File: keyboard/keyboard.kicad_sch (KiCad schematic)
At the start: 61 parts, among them J1 Conn_02x12_Odd_Even, SW1 true video, SW10 8, SW11 9, SW12 0, SW13 Break, SW14 delete, SW15 q, SW16 w, SW17 e, SW18 r, SW19 t, SW2 inverted video, SW20 y, SW21 u, SW22 i, SW23 o, SW24 p, SW25 graph, SW26 extended mode, SW27 edit, SW28 a, SW29 s, SW3 1, SW30 d, SW31 f, SW32 g, SW33 h, SW34 j, SW35 k, SW36 l, SW37 enter, SW38 caps shift left, SW39 caps lock, SW4 2, SW40 z, SW41 x, SW42 c, SW43 v, SW44 b, SW45 n, SW46 m, SW47 dot, SW48 caps shift right, SW49 symbol shift left, SW5 3, SW50 semicolon, SW51 quotes, SW52 left, SW53 right, SW54 left space, SW55 right space, SW56 up, SW57 down, SW58 comma, SW59 symbol shift right, SW6 4, SW60 rus-lat, SW7 5, SW8 6, SW9 7

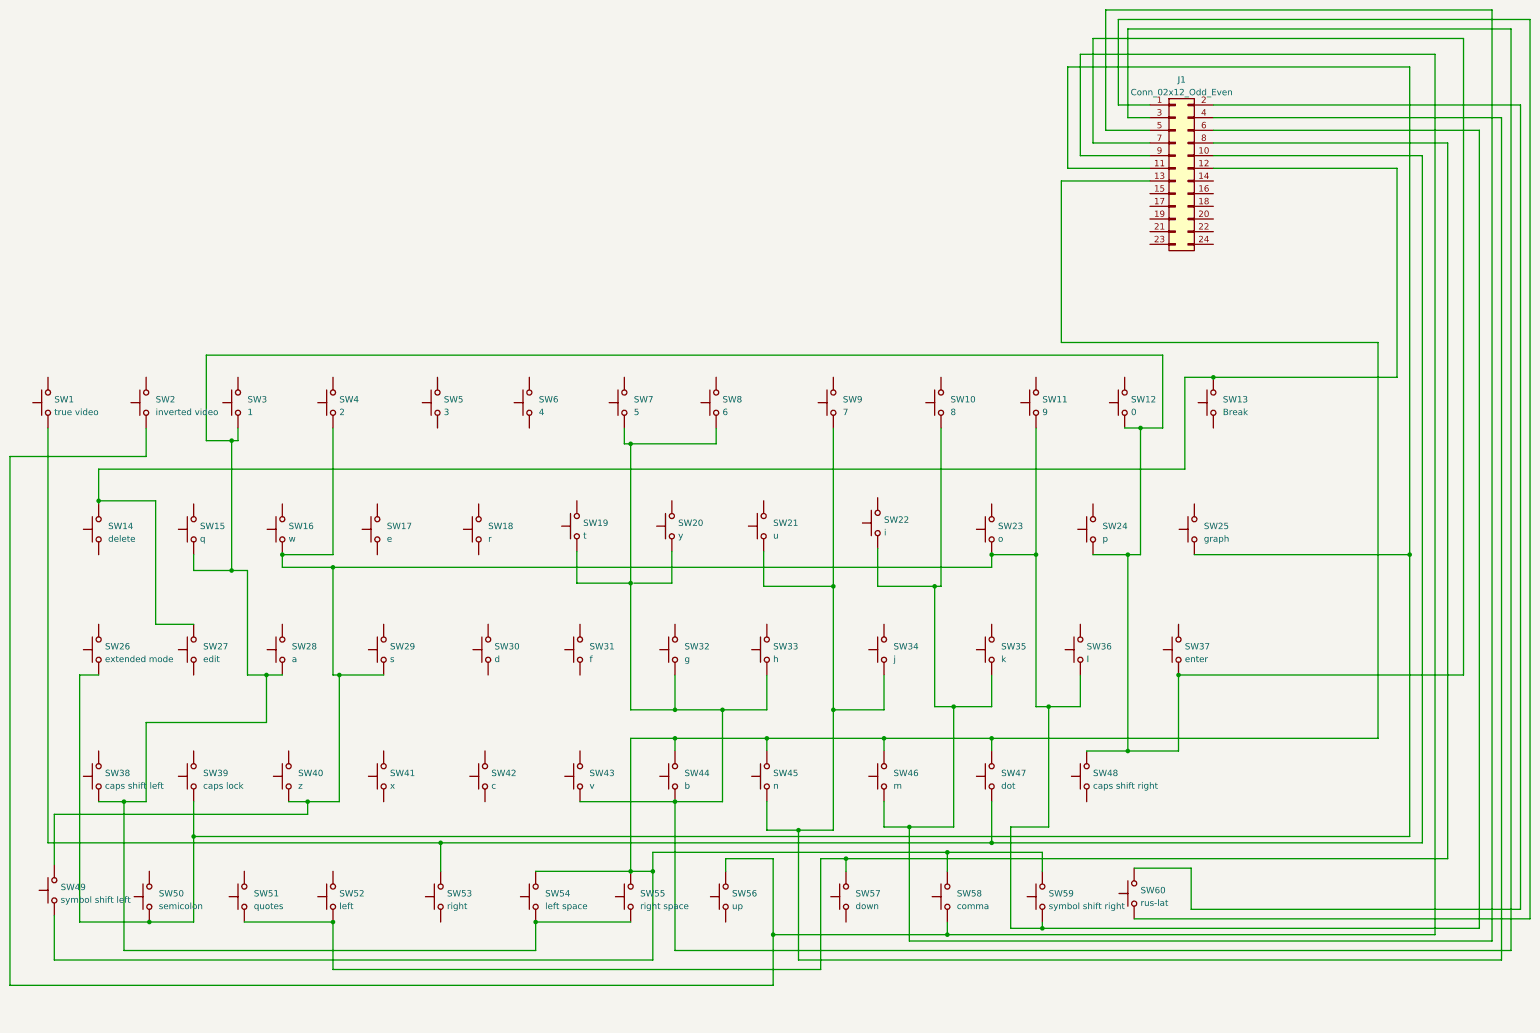
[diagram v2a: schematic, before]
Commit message: Late night update
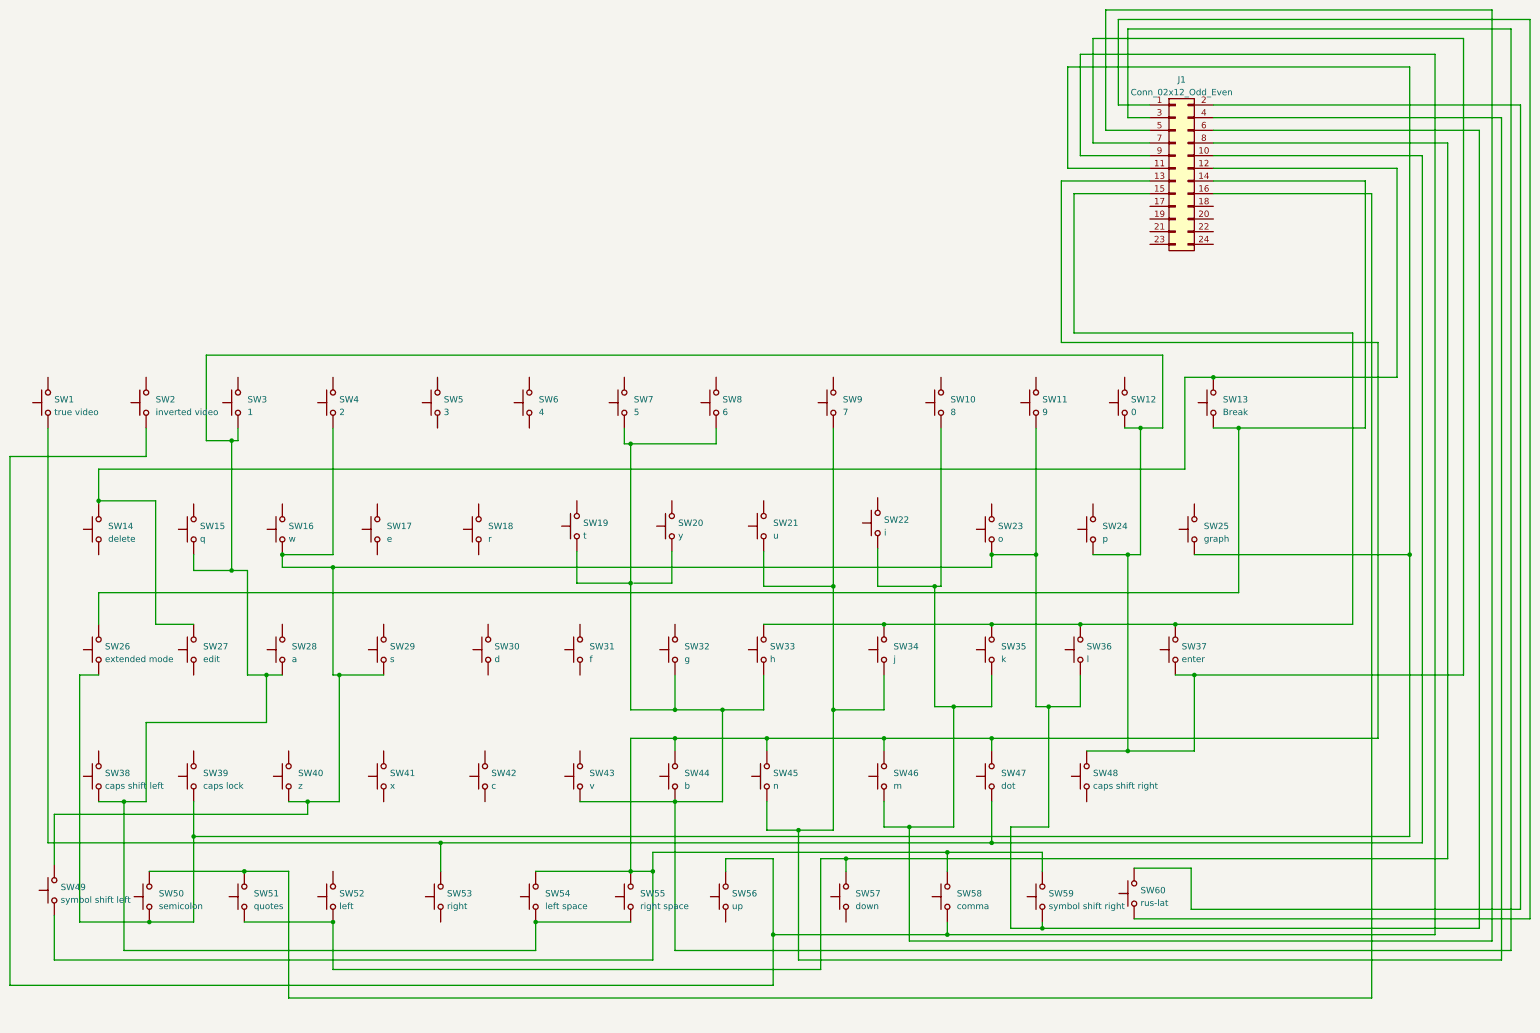
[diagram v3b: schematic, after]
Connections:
- net at SW35.2: now also J1.15 (Pin_15), SW33.2, SW34.2, SW36.2, SW37.2
- net at SW50.2: now also J1.16 (Pin_16), SW51.2
- net at SW26.2: now also J1.14 (Pin_14), SW13.1
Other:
- moved on the sheet: SW33, SW37
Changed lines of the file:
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@@
   (junction (at 204.47 189.23) (diameter 0) (color 0 0 0 0)
   )
+  (junction (at 127 189.23) (diameter 0) (color 0 0 0 0)
+  )
   (junction (at 360.68 125.73) (diameter 0) (color 0 0 0 0)
   )
@@
   (junction (at 222.885 156.845) (diameter 0) (color 0 0 0 0)
   )
+  (junction (at 276.86 139.7) (diameter 0) (color 0 0 0 0)
+  )
   (junction (at 321.31 90.17) (diameter 0) (color 0 0 0 0)
   )
   (junction (at 247.65 186.69) (diameter 0) (color 0 0 0 0)
   )
-  (junction (at 314.325 149.86) (diameter 0) (color 0 0 0 0)
+  (junction (at 317.5 149.86) (diameter 0) (color 0 0 0 0)
   )
   (junction (at 233.045 201.93) (diameter 0) (color 0 0 0 0)
@@
   (junction (at 208.915 189.23) (diameter 0) (color 0 0 0 0)
   )
+  (junction (at 255.27 139.7) (diameter 0) (color 0 0 0 0)
+  )
   (junction (at 231.775 162.56) (diameter 0) (color 0 0 0 0)
   )
@@
   (junction (at 131.445 149.86) (diameter 0) (color 0 0 0 0)
   )
+  (junction (at 313.69 139.7) (diameter 0) (color 0 0 0 0)
+  )
   (junction (at 144.78 128.27) (diameter 0) (color 0 0 0 0)
   )
@@
   (junction (at 204.47 131.445) (diameter 0) (color 0 0 0 0)
   )
+  (junction (at 326.39 100.33) (diameter 0) (color 0 0 0 0)
+  )
   (junction (at 124.46 102.87) (diameter 0) (color 0 0 0 0)
   )
   (junction (at 144.78 199.39) (diameter 0) (color 0 0 0 0)
   )
+  (junction (at 294.64 139.7) (diameter 0) (color 0 0 0 0)
+  )
   (junction (at 134.62 125.73) (diameter 0) (color 0 0 0 0)
   )
@@
     (stroke (width 0) (type default))
   )
+  (wire (pts (xy 351.79 100.33) (xy 326.39 100.33))
+    (stroke (width 0) (type default))
+  )
   (wire (pts (xy 139.7 175.26) (xy 146.05 175.26))
     (stroke (width 0) (type default))
@@
     (stroke (width 0) (type default))
   )
+  (wire (pts (xy 326.39 133.35) (xy 97.79 133.35))
+    (stroke (width 0) (type default))
+  )
   (wire (pts (xy 260.35 203.2) (xy 260.35 180.34))
     (stroke (width 0) (type default))
@@
     (stroke (width 0) (type default))
   )
+  (wire (pts (xy 255.27 139.7) (xy 276.86 139.7))
+    (stroke (width 0) (type default))
+  )
   (wire (pts (xy 119.38 102.87) (xy 124.46 102.87))
     (stroke (width 0) (type default))
@@
     (stroke (width 0) (type default))
   )
+  (wire (pts (xy 231.14 139.7) (xy 255.27 139.7))
+    (stroke (width 0) (type default))
+  )
+  (wire (pts (xy 321.31 50.8) (xy 351.79 50.8))
+    (stroke (width 0) (type default))
+  )
   (wire (pts (xy 124.46 128.905) (xy 127.635 128.905))
     (stroke (width 0) (type default))
@@
     (stroke (width 0) (type default))
   )
-  (wire (pts (xy 314.325 165.1) (xy 314.325 149.86))
+  (wire (pts (xy 317.5 165.1) (xy 317.5 149.86))
     (stroke (width 0) (type default))
   )
@@
     (stroke (width 0) (type default))
   )
+  (wire (pts (xy 135.89 214.63) (xy 135.89 189.23))
+    (stroke (width 0) (type default))
+  )
   (wire (pts (xy 102.87 175.26) (xy 102.87 205.105))
     (stroke (width 0) (type default))
@@
     (stroke (width 0) (type default))
   )
-  (wire (pts (xy 222.885 156.845) (xy 231.775 156.845))
-    (stroke (width 0) (type default))
-  )
-  (wire (pts (xy 231.775 156.845) (xy 231.775 149.86))
+  (wire (pts (xy 222.885 156.845) (xy 231.14 156.845))
+    (stroke (width 0) (type default))
+  )
+  (wire (pts (xy 231.14 156.845) (xy 231.14 149.86))
     (stroke (width 0) (type default))
   )
@@
     (stroke (width 0) (type default))
   )
+  (wire (pts (xy 308.61 53.34) (xy 293.37 53.34))
+    (stroke (width 0) (type default))
+  )
   (wire (pts (xy 292.1 27.94) (xy 360.68 27.94))
     (stroke (width 0) (type default))
@@
     (stroke (width 0) (type default))
   )
+  (wire (pts (xy 351.79 50.8) (xy 351.79 100.33))
+    (stroke (width 0) (type default))
+  )
   (wire (pts (xy 245.11 180.975) (xy 245.11 156.845))
     (stroke (width 0) (type default))
@@
     (stroke (width 0) (type default))
   )
+  (wire (pts (xy 326.39 100.33) (xy 326.39 133.35))
+    (stroke (width 0) (type default))
+  )
   (wire (pts (xy 363.22 183.515) (xy 276.86 183.515))
     (stroke (width 0) (type default))
   )
+  (wire (pts (xy 321.31 53.34) (xy 353.06 53.34))
+    (stroke (width 0) (type default))
+  )
   (wire (pts (xy 204.47 103.505) (xy 221.615 103.505))
     (stroke (width 0) (type default))
@@
     (stroke (width 0) (type default))
   )
-  (wire (pts (xy 304.165 165.1) (xy 314.325 165.1))
+  (wire (pts (xy 304.165 165.1) (xy 317.5 165.1))
     (stroke (width 0) (type default))
   )
@@
     (stroke (width 0) (type default))
   )
-  (wire (pts (xy 371.475 149.86) (xy 314.325 149.86))
+  (wire (pts (xy 371.475 149.86) (xy 317.5 149.86))
     (stroke (width 0) (type default))
   )
@@
     (stroke (width 0) (type default))
   )
+  (wire (pts (xy 353.06 214.63) (xy 135.89 214.63))
+    (stroke (width 0) (type default))
+  )
   (wire (pts (xy 134.62 125.73) (xy 134.62 128.27))
     (stroke (width 0) (type default))
@@
     (stroke (width 0) (type default))
   )
+  (wire (pts (xy 353.06 53.34) (xy 353.06 214.63))
+    (stroke (width 0) (type default))
+  )
   (wire (pts (xy 116.84 182.245) (xy 116.84 175.26))
     (stroke (width 0) (type default))
@@
     (stroke (width 0) (type default))
   )
+  (wire (pts (xy 293.37 53.34) (xy 293.37 81.28))
+    (stroke (width 0) (type default))
+  )
   (wire (pts (xy 144.78 199.39) (xy 144.78 208.915))
     (stroke (width 0) (type default))
   )
+  (wire (pts (xy 135.89 189.23) (xy 127 189.23))
+    (stroke (width 0) (type default))
+  )
   (wire (pts (xy 116.84 182.245) (xy 116.84 199.39))
     (stroke (width 0) (type default))
@@
     (stroke (width 0) (type default))
   )
+  (wire (pts (xy 97.79 133.35) (xy 97.79 139.7))
+    (stroke (width 0) (type default))
+  )
+  (wire (pts (xy 276.86 139.7) (xy 294.64 139.7))
+    (stroke (width 0) (type default))
+  )
   (wire (pts (xy 204.47 103.505) (xy 203.2 103.505))
     (stroke (width 0) (type default))
@@
     (stroke (width 0) (type default))
   )
+  (wire (pts (xy 349.25 139.7) (xy 313.69 139.7))
+    (stroke (width 0) (type default))
+  )
   (wire (pts (xy 231.14 132.08) (xy 231.14 125.095))
     (stroke (width 0) (type default))
@@
     (stroke (width 0) (type default))
   )
+  (wire (pts (xy 313.69 149.86) (xy 317.5 149.86))
+    (stroke (width 0) (type default))
+  )
   (wire (pts (xy 116.84 139.7) (xy 109.22 139.7))
     (stroke (width 0) (type default))
@@
     (stroke (width 0) (type default))
   )
+  (wire (pts (xy 293.37 81.28) (xy 349.25 81.28))
+    (stroke (width 0) (type default))
+  )
   (wire (pts (xy 87.63 183.515) (xy 87.63 100.33))
     (stroke (width 0) (type default))
@@
     (stroke (width 0) (type default))
   )
+  (wire (pts (xy 313.69 139.7) (xy 294.64 139.7))
+    (stroke (width 0) (type default))
+  )
+  (wire (pts (xy 326.39 100.33) (xy 321.31 100.33))
+    (stroke (width 0) (type default))
+  )
   (wire (pts (xy 213.36 175.26) (xy 213.36 205.105))
     (stroke (width 0) (type default))
   )
+  (wire (pts (xy 349.25 81.28) (xy 349.25 139.7))
+    (stroke (width 0) (type default))
+  )
   (wire (pts (xy 267.97 185.42) (xy 287.02 185.42))
     (stroke (width 0) (type default))
@@
     (stroke (width 0) (type default))
   )
+  (wire (pts (xy 107.95 189.23) (xy 127 189.23))
+    (stroke (width 0) (type default))
+  )
   (wire (pts (xy 185.42 199.39) (xy 204.47 199.39))
     (stroke (width 0) (type default))
@@
     )
   )
-  (symbol (lib_id "Switch:SW_Push") (at 231.775 144.78 90) (unit 1)
-    (in_bom yes) (on_board yes) (dnp no) (fields_autoplaced)
-    (property "Reference" "SW33" (at 233.045 144.145 90)
-      (effects (font (size 1.27 1.27)) (justify right))
-    )
-    (property "Value" "h" (at 233.045 146.685 90)
-      (effects (font (size 1.27 1.27)) (justify right))
-    )
-    (property "Footprint" "Library:key" (at 226.695 144.78 0)
-      (effects (font (size 1.27 1.27)) hide)
-    )
-    (property "Datasheet" "~" (at 226.695 144.78 0)
+  (symbol (lib_id "Switch:SW_Push") (at 231.14 144.78 90) (unit 1)
+    (in_bom yes) (on_board yes) (dnp no) (fields_autoplaced)
+    (property "Reference" "SW33" (at 232.41 144.145 90)
+      (effects (font (size 1.27 1.27)) (justify right))
+    )
+    (property "Value" "h" (at 232.41 146.685 90)
+      (effects (font (size 1.27 1.27)) (justify right))
+    )
+    (property "Footprint" "Library:key" (at 226.06 144.78 0)
+      (effects (font (size 1.27 1.27)) hide)
+    )
+    (property "Datasheet" "~" (at 226.06 144.78 0)
       (effects (font (size 1.27 1.27)) hide)
     )
@@
     )
   )
-  (symbol (lib_id "Switch:SW_Push") (at 314.325 144.78 90) (unit 1)
-    (in_bom yes) (on_board yes) (dnp no) (fields_autoplaced)
-    (property "Reference" "SW37" (at 315.595 144.145 90)
-      (effects (font (size 1.27 1.27)) (justify right))
-    )
-    (property "Value" "enter" (at 315.595 146.685 90)
-      (effects (font (size 1.27 1.27)) (justify right))
-    )
-    (property "Footprint" "Library:key" (at 309.245 144.78 0)
-      (effects (font (size 1.27 1.27)) hide)
-    )
-    (property "Datasheet" "~" (at 309.245 144.78 0)
-      (effects (font (size 1.27 1.27)) hide)
-    )
+  (symbol (lib_id "Switch:SW_Push") (at 313.69 144.78 90) (unit 1)
+    (in_bom yes) (on_board yes) (dnp no) (fields_autoplaced)
+    (property "Reference" "SW37" (at 314.96 144.145 90)
+      (effects (font (size 1.27 1.27)) (justify right))
+    )
+    (property "Value" "enter" (at 314.96 146.685 90)
+      (effects (font (size 1.27 1.27)) (justify right))
+    )
+    (property "Footprint" "Library:key" (at 308.61 144.78 0)
+      (effects (font (size 1.27 1.27)) hide)
+    )
+    (property "Datasheet" "~" (at 308.61 144.78 0)
+      (effects (font (size 1.27 1.27)) hide)
+    )

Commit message: Tracing finished
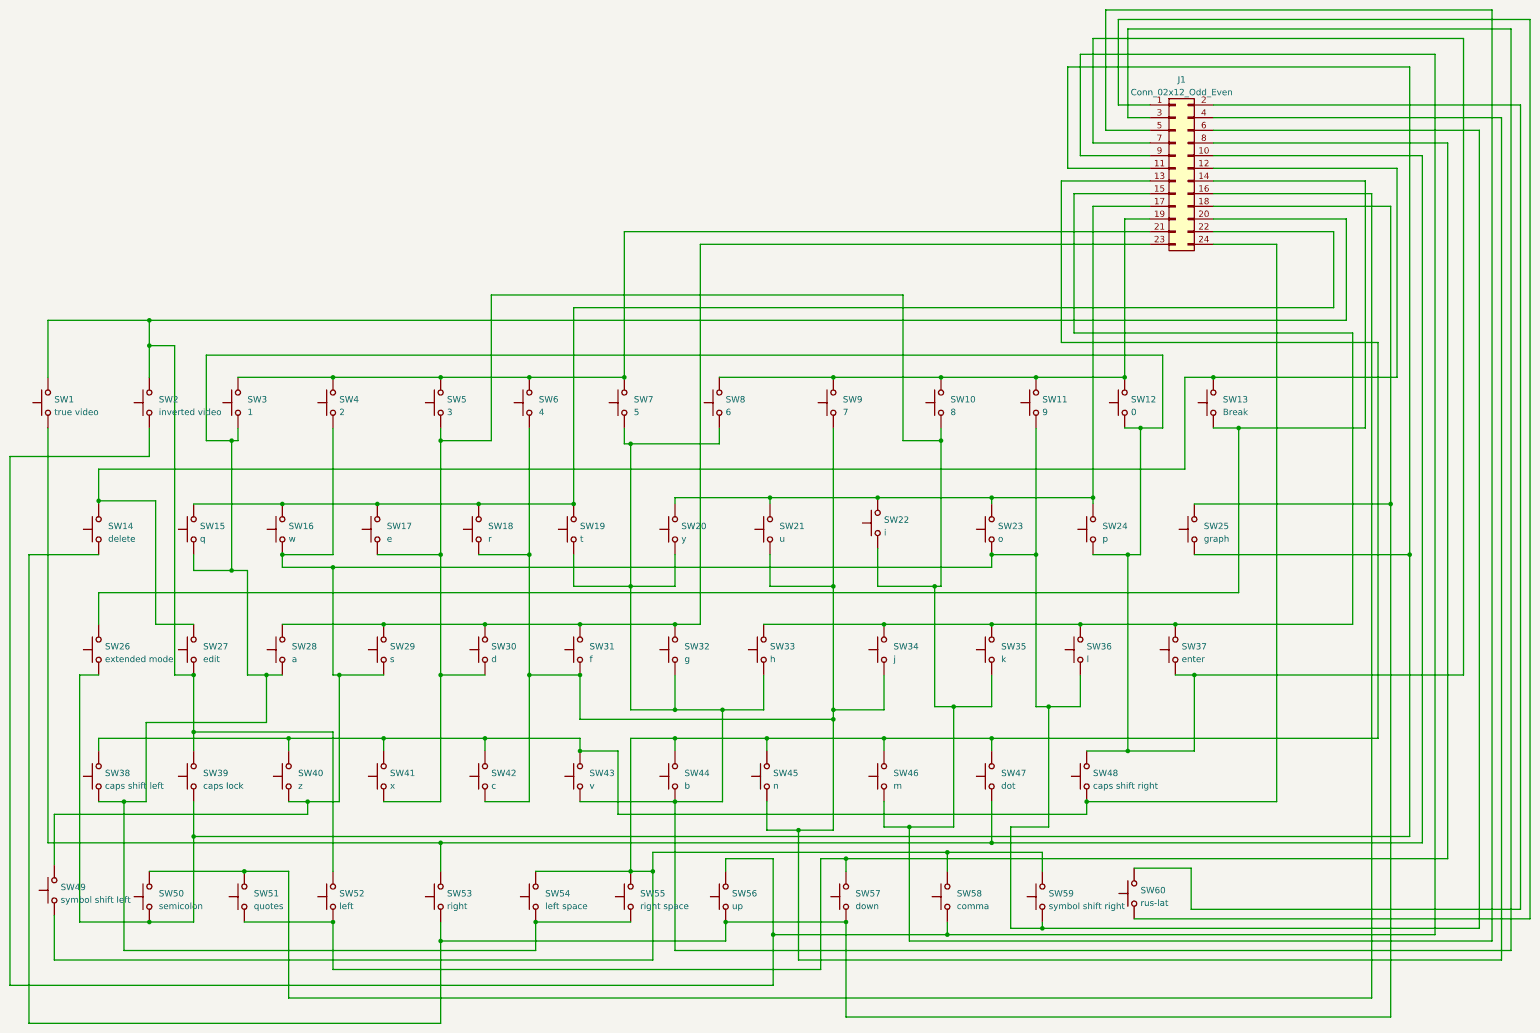
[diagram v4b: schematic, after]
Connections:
- net at SW31.1: now also J1.4 (Pin_4), SW18.1, SW21.1, SW34.1, SW42.1, SW45.1, SW6.1, SW9.1
- net at SW31.2: now also J1.23 (Pin_23), SW28.2, SW29.2, SW30.2, SW32.2
- net at SW57.1: now also J1.18 (Pin_18), SW14.1, SW25.2, SW53.1, SW56.1
- net at SW15.2: now also J1.22 (Pin_22), SW16.2, SW17.2, SW18.2, SW19.2
- net at J1.5 (Pin_5), SW10.1, SW22.1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: now also SW17.1, SW30.1, SW41.1, SW5.1
- net at SW40.2: now also J1.24 (Pin_24), SW38.2, SW41.2, SW42.2, SW43.2, SW48.1
- net at J1.3 (Pin_3), SW19.1, SW32.1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: now also SW20.1
- net at SW1.2: now also J1.20 (Pin_20), SW2.2, SW27.1, SW39.2, SW52.2
- net at SW20.2: now also J1.17 (Pin_17), SW21.2, SW22.2, SW23.2, SW24.2
- net at SW8.2: now also J1.19 (Pin_19), SW10.2, SW11.2, SW12.2, SW9.2
- net at SW5.2: now also J1.21 (Pin_21), SW3.2, SW4.2, SW6.2, SW7.2
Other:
- moved on the sheet: SW19, SW2, SW20, SW21, SW30, SW5, SW8
